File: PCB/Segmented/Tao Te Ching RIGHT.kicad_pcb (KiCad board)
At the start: 2 copper layers, 138.2 x 89.7 mm, 49 parts, among them SW25 SW_Push_45deg, SW26 SW_Push_45deg, SW27 SW_Push_45deg, SW28 SW_Push_45deg, SW29 SW_Push_45deg, SW30 SW_Push_45deg, SW31 SW_Push_45deg, SW32 SW_Push_45deg, SW33 SW_Push_45deg, SW34 SW_Push_45deg, SW35 SW_Push_45deg, SW36 SW_Push_45deg, SW37 SW_Push_45deg, SW38 SW_Push_45deg, SW39 SW_Push_45deg, SW40 SW_Push_45deg, SW41 SW_Push_45deg, SW42 SW_Push_45deg, SW43 SW_Push_45deg, SW44 SW_Push_45deg, SW45 SW_Push_45deg, SW46 SW_Push_45deg, SW47 SW_Push_45deg, SW48 SW_Push_45deg, U2 XIAO-nRF52840-DIP

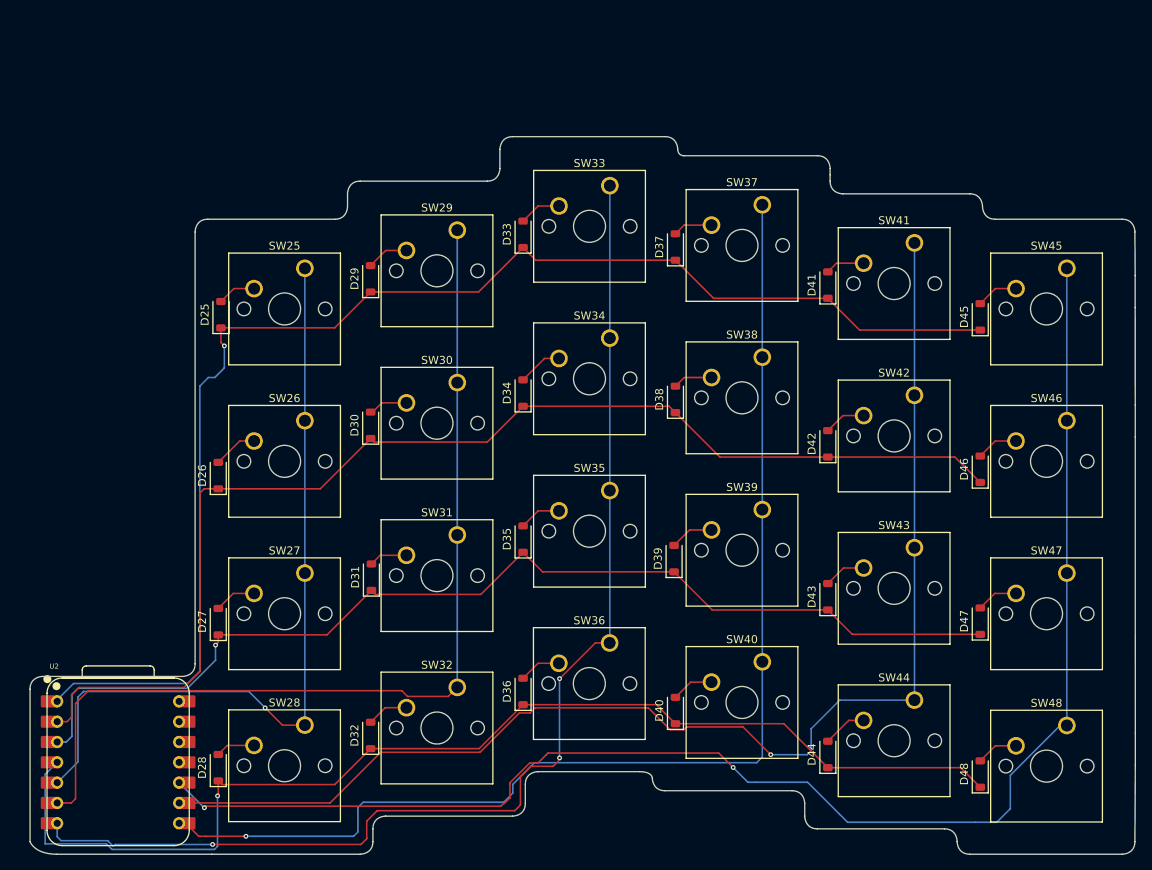
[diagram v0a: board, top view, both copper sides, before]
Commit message: Reworked Case and images
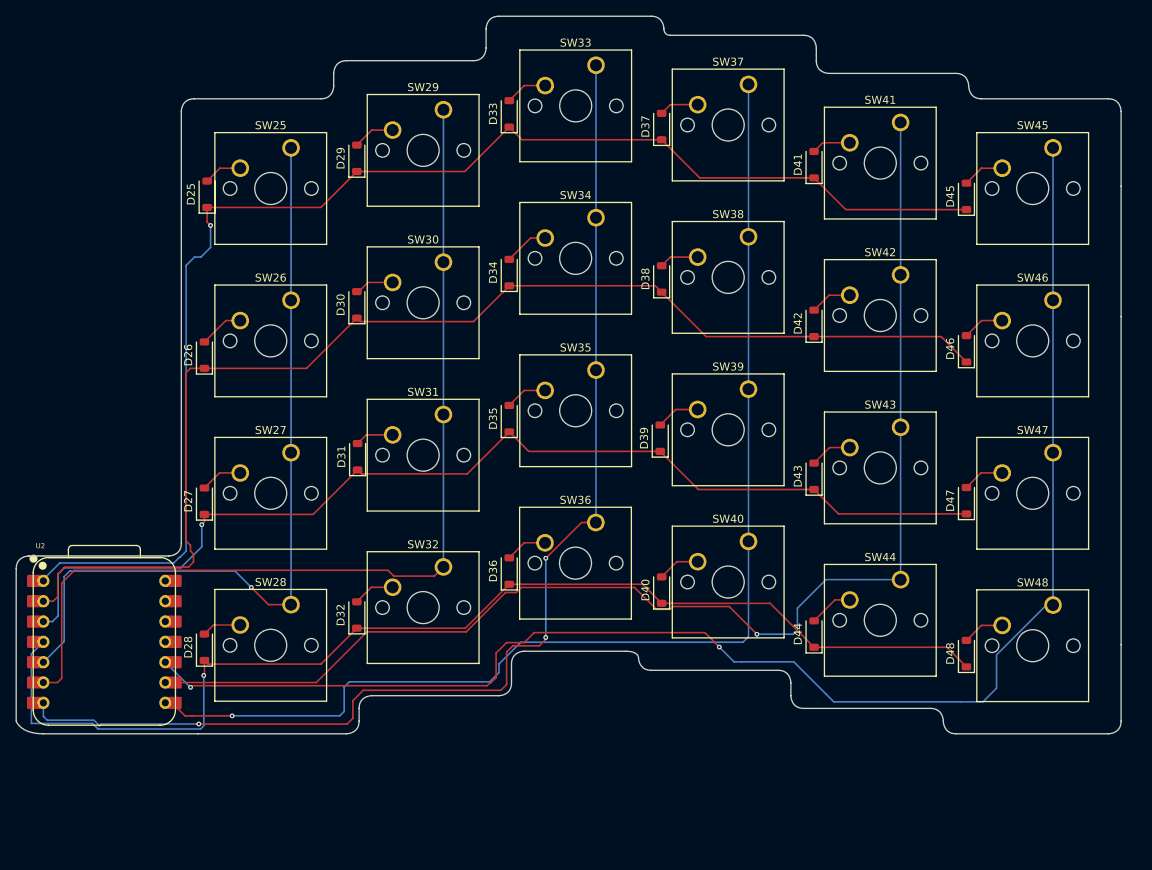
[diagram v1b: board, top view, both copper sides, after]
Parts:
- moved D26 15.2 mm to (91.9, 76.1)
- moved D41 15.2 mm to (168.1, 52.3)
- moved D42 15.2 mm to (168.1, 72.1)
- moved D43 15.2 mm to (168.1, 91.2)
- moved D44 15.2 mm to (168.1, 110.9)
- moved D45 15.2 mm to (187.2, 56.2)
- moved D46 15.2 mm to (187.2, 75.3)
- moved D48 15.2 mm to (187.2, 113.4)
- moved SW27 15.2 mm to (102.7, 88.3)
- moved SW28 15.2 mm to (102.7, 107.3)
- moved SW31 15.2 mm to (121.8, 83.5)
- moved SW32 15.2 mm to (121.8, 102.5)
- moved SW44 15.2 mm to (178.9, 104.1)
- moved SW47 15.2 mm to (198.0, 88.3)
- moved SW48 15.2 mm to (198.0, 107.3)
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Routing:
- net Row5: track 150.7 -> 152.8 mm
- net Col11: track 184.4 -> 185.1 mm
- net Row6: track 134.6 -> 135.1 mm
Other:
- board size 138.2 x 89.7 mm -> 138.1 x 89.7 mm
